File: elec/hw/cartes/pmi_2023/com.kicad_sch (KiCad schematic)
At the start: 39 parts, among them J7 USB4105-GF-A-060, Q4 SI2310, SW10 TSB001A3526A02, SW7 MSS12C02LS-BB2.0, U32 ESP32-S3-WROOM-1

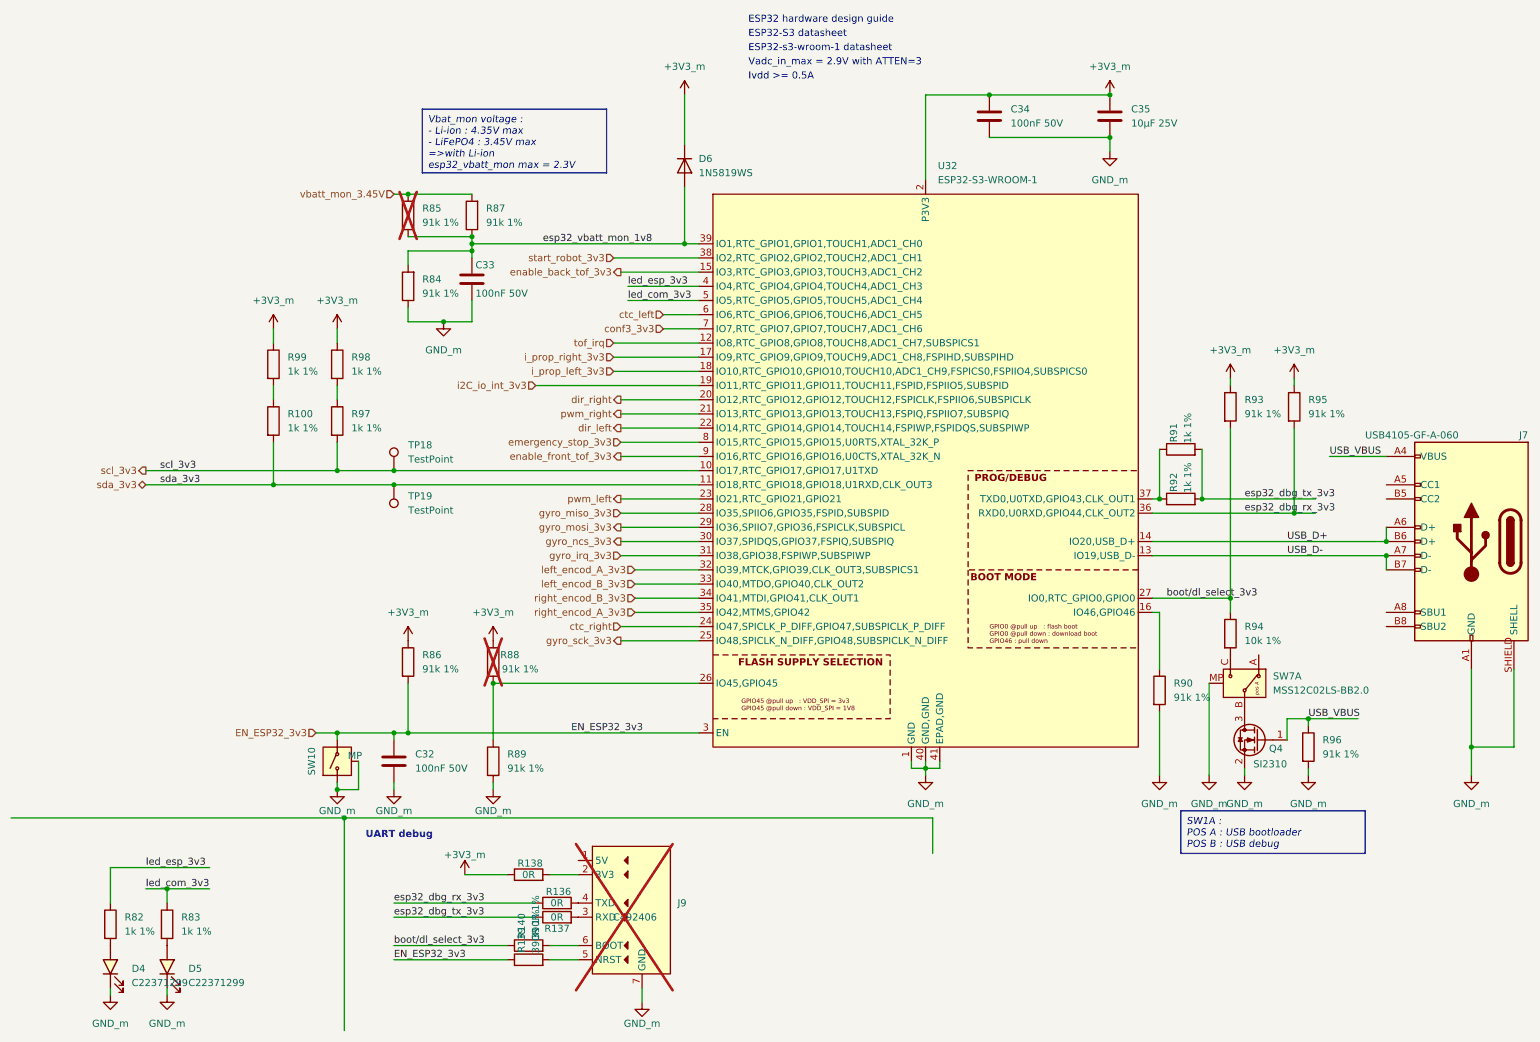
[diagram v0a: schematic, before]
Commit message: pmi board V2, ready for review
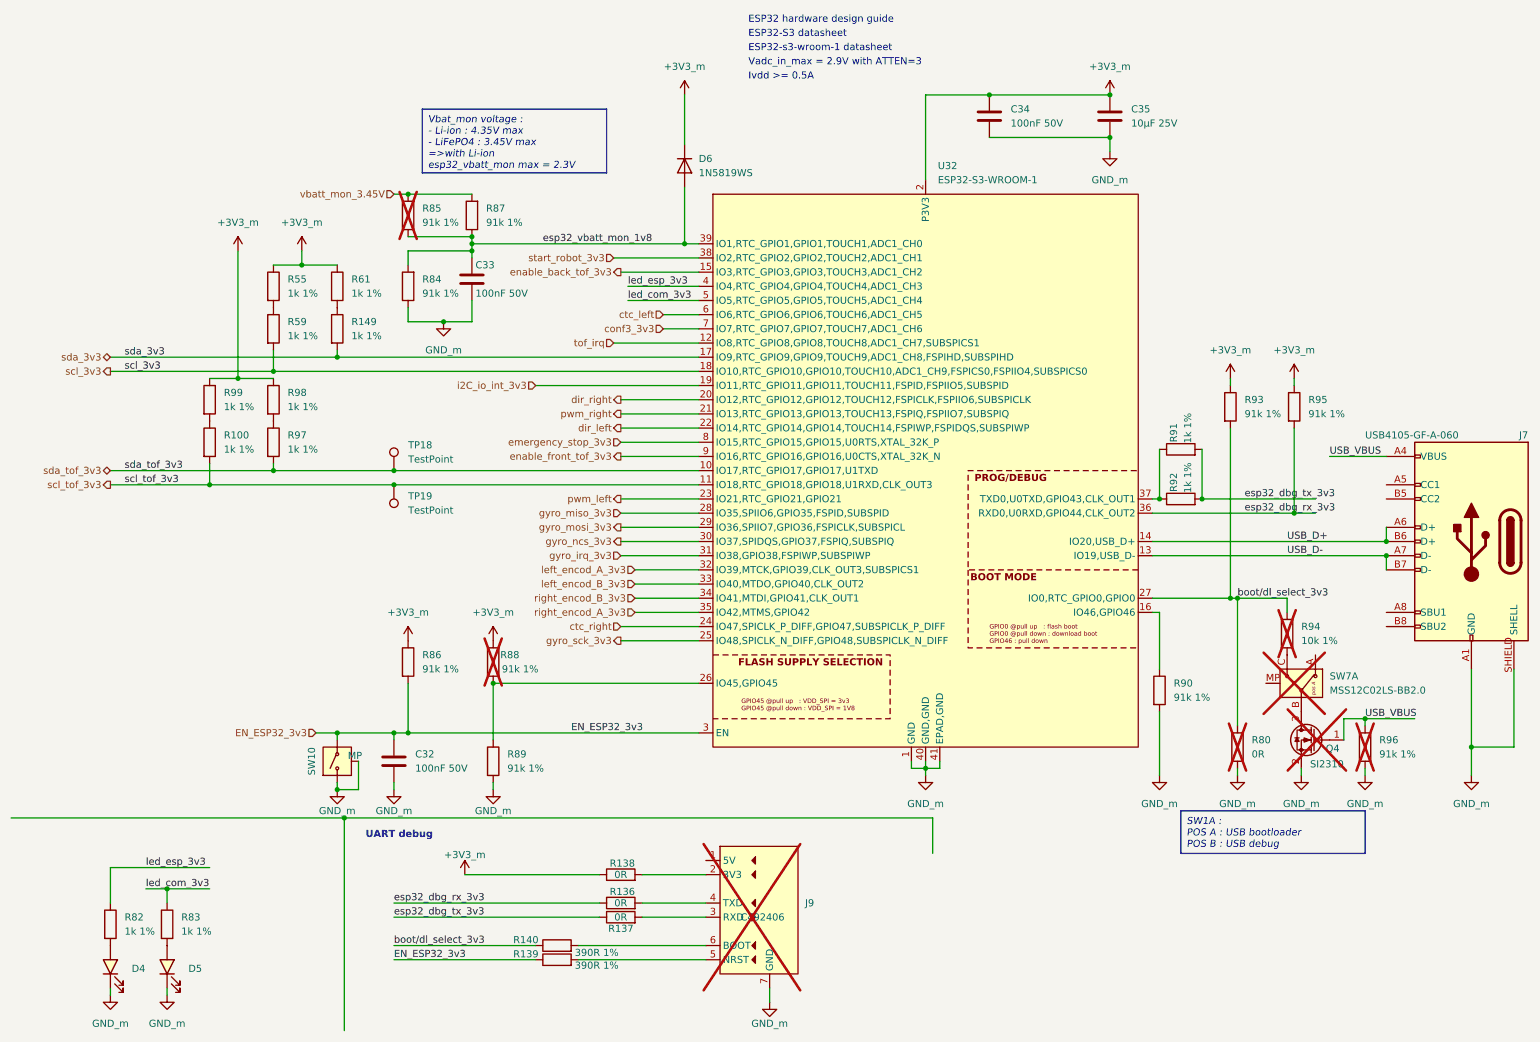
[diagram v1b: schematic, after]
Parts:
- added R149, R55, R59, R61: 1k 1%, cocotter_resistor:r0603_reflow, symbol cocotter_resistors:R_1k_0603_1%
- added R80: 0R, cocotter_resistor:r0603_reflow, symbol cocotter_resistors:R_0R_0603
- Q4, R94, R96, SW7: now not fitted
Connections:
- net i_prop_left_3v3 is gone; now on net scl_3v3: U32.18 (IO10,RTC_GPIO10,GPIO10,TOUCH10,ADC1_CH9,FSPICS0,FSPIIO4,SUBSPICS0)
- net i_prop_right_3v3 is gone; now on net sda_3v3: U32.17 (IO9,RTC_GPIO9,GPIO9,TOUCH9,ADC1_CH8,FSPIHD,SUBSPIHD)
- net +3V3_m: now also R55.1, R61.1
- net GND_m: now also R80.2; no longer SW7.MP
- net boot/dl_select_3v3: now also R80.1
- net scl_3v3: now also R59.2; no longer R97.2, TP18.1, U32.10 (IO17,RTC_GPIO17,GPIO17,U1TXD)
- net sda_3v3: now also R149.2; no longer R100.2, TP19.1, U32.11 (IO18,RTC_GPIO18,GPIO18,U1RXD,CLK_OUT3)
- new net: R55.2, R59.1
- new net: R149.1, R61.2
- new net scl_tof_3v3: R100.2, TP19.1, U32.11 (IO18,RTC_GPIO18,GPIO18,U1RXD,CLK_OUT3)
- new net sda_tof_3v3: R97.2, TP18.1, U32.10 (IO17,RTC_GPIO17,GPIO17,U1TXD)
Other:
- moved on the sheet: J9, R100, R136, R137, R138, R139, R140, R97, R98, R99
